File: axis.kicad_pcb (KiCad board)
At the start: 4 copper layers, 66 x 18 mm, 46 parts, among them J101 CORTEX-DEBUG, J102 JAE_DX07S016JA3, SW101 SW_Push, SW102 SW_Push, U101 TPS78433QWDRBRQ1, U102 ATSAMD51G, U103 BMM150, U104 BHI160, Y101 32k768

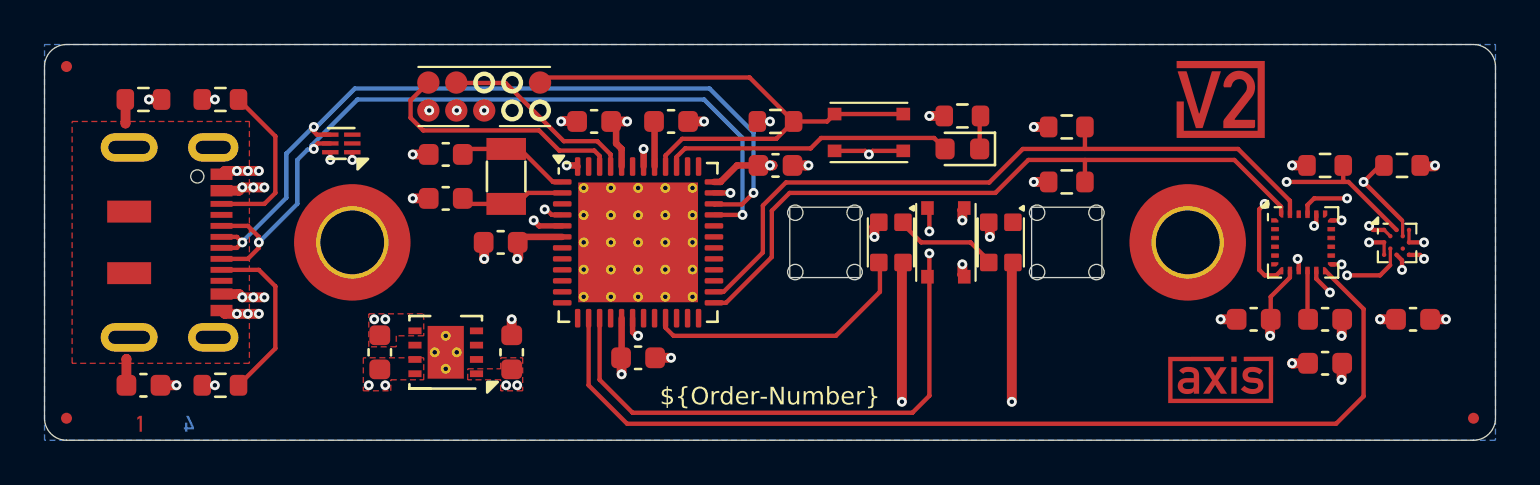
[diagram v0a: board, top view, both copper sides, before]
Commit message: Update
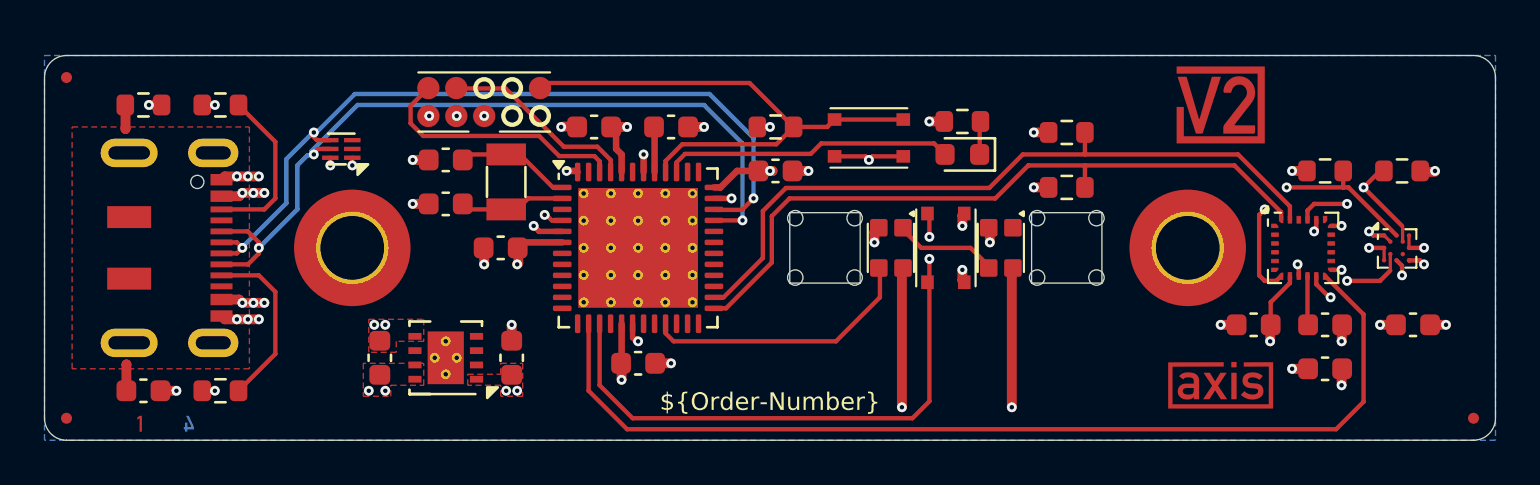
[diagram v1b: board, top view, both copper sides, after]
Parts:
- moved FID102 0.50 mm to (118.0, 98.5)
- moved C101 0.25 mm to (145.5, 100.8)
- moved C102 0.25 mm to (150.2, 102.8)
- moved C103 0.25 mm to (142.0, 100.8)
- moved C104 0.25 mm to (144.0, 111.5)
- moved C105 0.25 mm to (137.8, 106.2)
- moved C106 0.25 mm to (132.2, 111.2)
- moved C107 0.25 mm to (138.2, 111.2)
- moved C108 0.25 mm to (135.2, 102.2)
- moved C109 0.25 mm to (135.2, 104.2)
- moved C110 0.25 mm to (121.5, 112.8)
- moved C111 0.25 mm to (172.0, 109.8)
- moved C112 0.25 mm to (175.2, 111.8)
- moved C113 0.25 mm to (179.2, 109.8)
- moved C114 0.25 mm to (175.2, 109.8)
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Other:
- board size 66 x 18 mm -> 66 x 17.5 mm
